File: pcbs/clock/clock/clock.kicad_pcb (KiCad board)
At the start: 2 copper layers, 90 parts, among them J1 USB_B_Micro, J2 CORTEX, Q1 BSS138, Q10 BSS138, Q11 BSS138, Q12 BSS138, Q2 BSS138, Q3 BSS138, Q4 BSS138, Q5 BSS138, Q6 BSS138, Q7 BSS138, Q8 BSS138, Q9 BSS138, SW1 SW_Push, U1 USBLC6-2SC6, U10 KCSC02-105, U11 KCSC02-105, U12 KCSC02-105, U13 KCSC02-105, U14 KCSC02-105, U15 KCSC02-105, U16 KCSC02-105, U2 AP2112K-3.3, U3 SAMD21Exx, U4 PCF85263ATT, U5 TCA6416APWR, U6 AT24CS01-SSHM, U7 KCSC02-105, U8 KCSC02-105, U9 KCSC02-105, Y1 32.768k

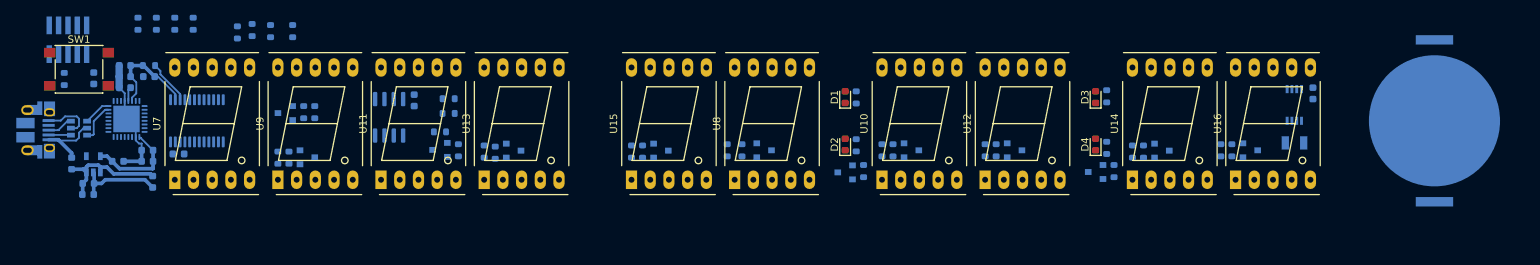
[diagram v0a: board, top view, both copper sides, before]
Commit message: Progress
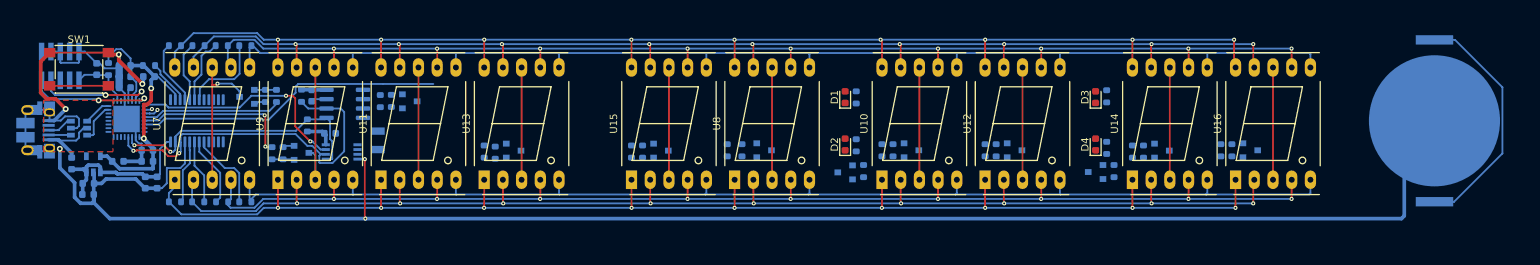
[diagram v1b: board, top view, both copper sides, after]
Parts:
- moved C10 133.5 mm to (98.1, 128.7), turned to 180 degrees
- moved U4 129.5 mm to (99.7, 131.2), turned to 180 degrees
- moved Y1 124.4 mm to (104.6, 129.7), turned to 270 degrees
- moved R16 28.2 mm to (86.6, 138.0), turned to 180 degrees
- moved R11 25.0 mm to (83.4, 138.0), turned to 180 degrees
- moved R13 24.3 mm to (77.0, 138.0), turned to 0 degrees
- moved R12 24.2 mm to (80.2, 138.0), turned to 0 degrees
- moved R37 20.0 mm to (94.2, 123.6), turned to 270 degrees
- moved R38 19.2 mm to (95.0, 127.6), turned to 90 degrees
- moved C14 13.9 mm to (95.6, 123.6)
- moved R15 13.1 mm to (77.0, 116.8), turned to 180 degrees
- moved R27 11.3 mm to (106.4, 124.3), turned to 270 degrees
- moved R9 9.83 mm to (83.4, 116.8), turned to 180 degrees
- moved R25 9.11 mm to (104.9, 124.3), turned to 90 degrees
- moved Q7 7.77 mm to (108.9, 124.3), turned to 0 degrees
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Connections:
- U3 pad 13: /CH1 -> /CH6
- U3 pad 14: /CH2 -> /CH7
- U3 pad 15: /CH3 -> /CH8
- U3 pad 16: /CH4 -> /CH9
- U3 pad 17: /CH5 -> /CH10
- U3 pad 4: /CH6 -> /CH1
- U3 pad 5: /CH7 -> /CH2
- U3 pad 6: /CH8 -> /CH3
- U3 pad 7: /CH9 -> /CH4
- U3 pad 8: /CH10 -> /CH5
- U5 pad 10: /Displays/SEG_G -> Net-(U5-Pad10)
- U5 pad 11: /Displays/SEG_DP -> Net-(U5-Pad11)
- U5 pad 17: Net-(U5-Pad17) -> /Displays/SEG_DP
- U5 pad 18: Net-(U5-Pad18) -> /Displays/SEG_C
- U5 pad 19: Net-(U5-Pad19) -> /Displays/SEG_D
- U5 pad 20: Net-(U5-Pad20) -> /Displays/SEG_E
- U5 pad 4: /Displays/SEG_A -> /Displays/SEG_G
- U5 pad 5: /Displays/SEG_B -> /Displays/SEG_F
- U5 pad 6: /Displays/SEG_C -> /Displays/SEG_A
- U5 pad 7: /Displays/SEG_D -> /Displays/SEG_B
- U5 pad 8: /Displays/SEG_E -> Net-(U5-Pad8)
- U5 pad 9: /Displays/SEG_F -> Net-(U5-Pad9)
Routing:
- net GND: track 35.3 -> 328.2 mm, vias 0 -> 6
- net /Displays/SEGE: track 0.00 -> 183.6 mm, vias 0 -> 9
- net /Displays/SEGG: track 0.00 -> 181.5 mm, vias 0 -> 9
- net /Displays/SEGD: track 0.00 -> 177.2 mm, vias 0 -> 9
- net /Displays/SEGF: track 0.00 -> 175.8 mm, vias 0 -> 9
- net /Displays/SEGC: track 0.00 -> 172.1 mm, vias 0 -> 9
- net /Displays/SEGA: track 0.00 -> 171.5 mm, vias 0 -> 9
- net /Displays/SEGDP: track 0.00 -> 165.7 mm
- net /Displays/SEGB: track 0.00 -> 165.0 mm
- net /SCL: track 0.00 -> 49.3 mm, vias 0 -> 2
- net /CH3: track 0.00 -> 42.1 mm
- net /SDA: track 0.00 -> 37.4 mm, vias 0 -> 2
- net Net-(BT1-Pad1): track 0.00 -> 32.8 mm
- net /CLKI: track 0.00 -> 30.8 mm, vias 0 -> 2
- net +3V3: track 26.7 -> 51.3 mm, vias 0 -> 2
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- added copper zone on F.Cu, net GND

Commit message: Progress
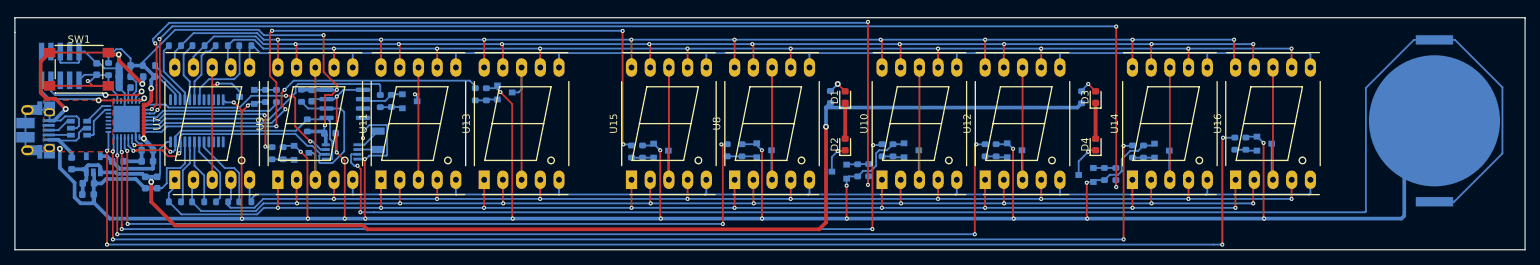
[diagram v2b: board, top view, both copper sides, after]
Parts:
- moved R31 8.02 mm to (119.3, 123.4)
- moved Q9 7.99 mm to (121.8, 123.2)
- moved R29 7.87 mm to (117.8, 123.4)
- moved R1 3.78 mm to (171.2, 133.7), turned to 90 degrees
- moved R5 3.76 mm to (204.8, 134.2), turned to 90 degrees
- moved R3 3.50 mm to (166.0, 123.8)
- moved R7 3.40 mm to (200.1, 123.8)
- moved Q12 2.10 mm to (224.9, 130.1)
- moved R34 2.10 mm to (220.9, 130.1)
- moved R36 2.10 mm to (222.4, 130.1)
- moved Q2 1.36 mm to (200.7, 134.3)
- moved R6 1.36 mm to (203.2, 134.2)
- moved Q1 0.81 mm to (167.2, 133.9)
- moved R2 0.81 mm to (169.7, 133.7)
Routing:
- net /CH10: track 0.00 -> 182.9 mm, vias 0 -> 4
- net GND: track 328.2 -> 508.6 mm, vias 6 -> 29
- net Net-(BT1-Pad1): track 32.8 -> 207.7 mm, vias 0 -> 2
- net /CH9: track 0.00 -> 165.1 mm, vias 0 -> 4
- net /DT2: track 1.97 -> 165.1 mm, vias 1 -> 4
- net +5V: track 22.7 -> 171.0 mm, vias 0 -> 2
- net /CH8: track 0.00 -> 143.1 mm, vias 0 -> 4
- net /DT1: track 1.04 -> 132.3 mm, vias 1 -> 4
- net /CH7: track 0.00 -> 127.1 mm, vias 0 -> 4
- net /CH6: track 0.00 -> 104.5 mm, vias 0 -> 4
- net /CH5: track 0.00 -> 95.9 mm, vias 0 -> 4
- net /CH4: track 0.00 -> 50.2 mm, vias 0 -> 2
- net +3V3: track 51.3 -> 95.2 mm, vias 2 -> 5
- net /CH3: track 42.1 -> 36.3 mm
- net Net-(Q12-Pad3): track 15.2 -> 20.2 mm
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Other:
- board outline added: 205 x 31.5 mm
